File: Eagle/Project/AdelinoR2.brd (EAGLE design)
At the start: 47 x 53.3 mm, 79 parts, among them J1 DC-044-A, J2 YELLOW-8P-2.54, J3 YELLOW-6P-2.54, J4 YELLOW-8P-2.54, J5 YELLOW-8P-2.54, J6 4P-2.0, J7 YELLOW-2X3P-2.54, J8 4P-2.0, Q1 NCE3407A, Q2 CJ2305, SW1 TS-1101F, U1 CJT1117-3.3-SOT223, U2 MP1496DJ-SOT23-8, U3 ESP-12F / OPL: 317060163 / SM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, U4 ATMEGA32U4-MUR-QFN44, U5 ATMEGA32U4-TQFP44, U6 ATECC608-SOIC8, X1 306010049_XTAL_16MHZ-3225_4P

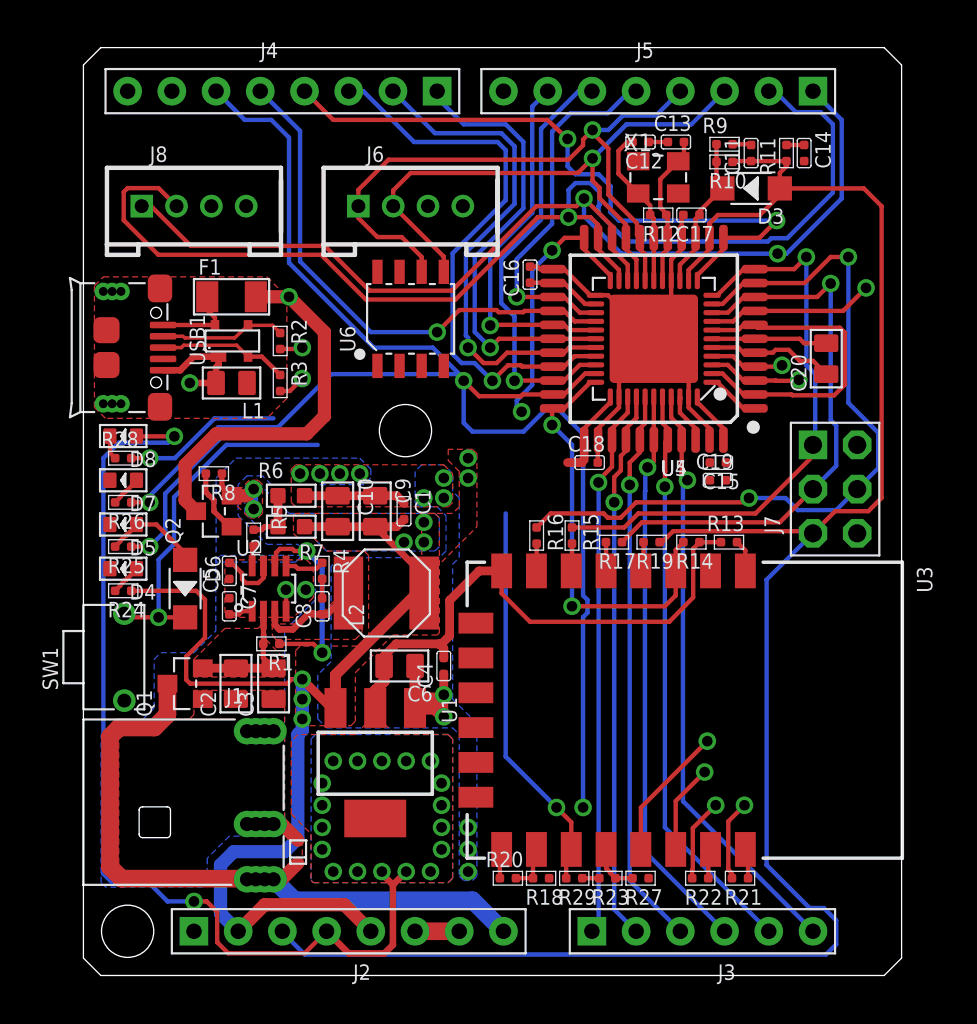
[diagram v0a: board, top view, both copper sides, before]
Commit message: Routing wip.
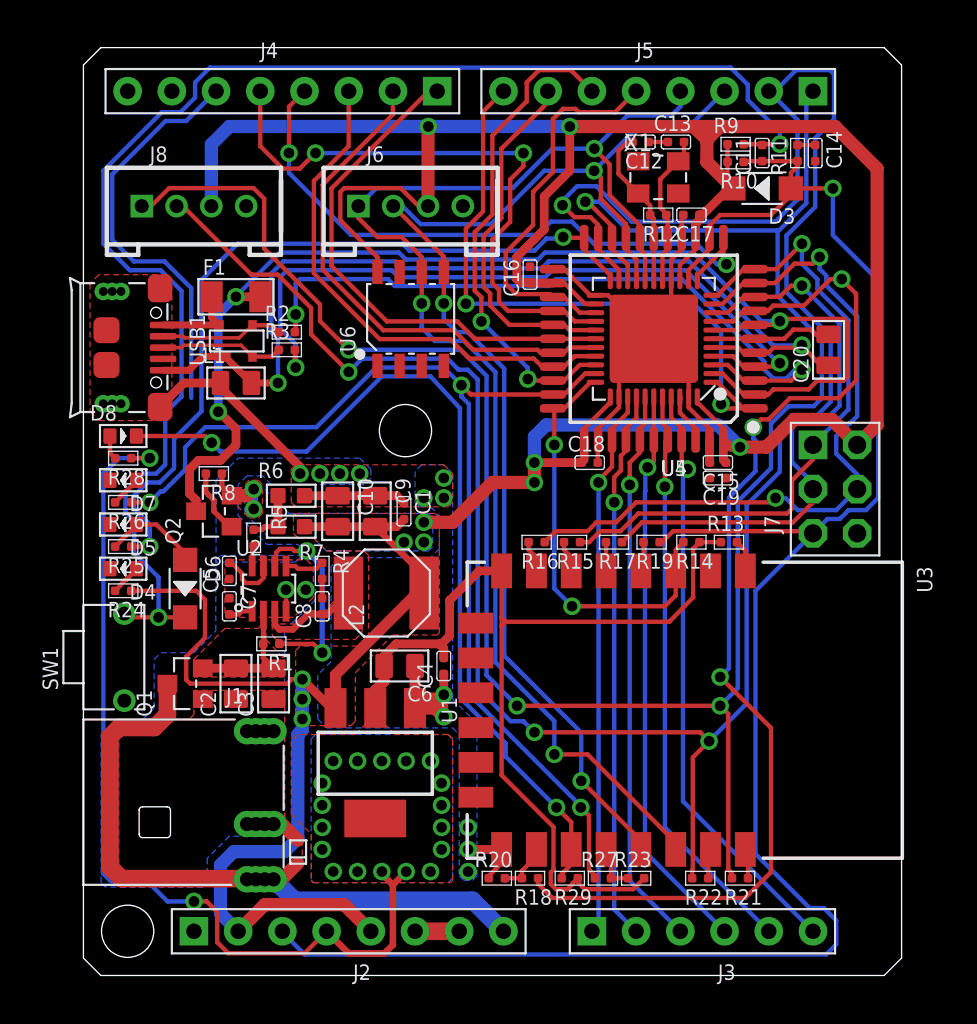
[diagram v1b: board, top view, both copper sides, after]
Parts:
- moved R27 2.16 mm to (29.8, 5.59), turned to 90 degrees
- moved R3 1.94 mm to (11.7, 35.9), turned to 90 degrees
- moved R23 1.65 mm to (31.8, 5.59), turned to 90 degrees
- moved R10 0.64 mm to (37.5, 46.7)
- moved R9 0.64 mm to (37.5, 47.8)
- moved R18 0.64 mm to (25.7, 5.59)
- moved R20 0.64 mm to (23.7, 5.59)
- moved R2 0.64 mm to (11.7, 37.0), turned to 90 degrees
- moved C11 0.63 mm to (39.0, 47.2)
- moved C14 0.63 mm to (42.0, 47.2)
- moved D3 0.63 mm to (39.0, 45.2)
- moved R11 0.63 mm to (41.0, 47.2)
- moved C20 0.52 mm to (42.8, 35.9)
- moved R15 0.38 mm to (28.1, 24.9), turned to 270 degrees
- moved R16 0.38 mm to (26.0, 24.9), turned to 270 degrees
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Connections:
- net +3V3: now also R28.1; no longer D8.+
- net GPIO2_LED: now also D8.-; no longer R28.2
- net N$4: now also D8.+, R28.2; no longer D8.-, R28.1
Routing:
- net +5V: track 92.1 -> 219.5 mm, vias 10 -> 13
- net PIN_D1: track 73.5 -> 140.7 mm, vias 2 -> 4
- net PIN_D0: track 64.9 -> 126.3 mm, vias 3 -> 4
- net RSTAT: track 21.4 -> 81.4 mm, vias 1 -> 2
- net AT_SS: track 9.64 -> 64.0 mm, vias 1 -> 3
- net UGND: track 13.9 -> 54.6 mm, vias 1 -> 2
- net D+: track 5.86 -> 42.2 mm
- net PIN_D3_SCL: track 43.1 -> 78.0 mm, vias 2 -> 3
- net PIN_D7: track 3.07 -> 37.7 mm, vias 0 -> 2
- net D-: track 6.68 -> 41.0 mm
- net PIN_D2_SDA: track 43.1 -> 73.1 mm, vias 2 -> 3
- net VUSB: track 41.0 -> 70.8 mm, vias 1 -> 3
- net +3V3: track 90.1 -> 109.9 mm
- net GPIO2_LED: track 31.8 -> 51.4 mm
- net ACT_LED: track 29.2 -> 45.2 mm, vias 3 -> 2
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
